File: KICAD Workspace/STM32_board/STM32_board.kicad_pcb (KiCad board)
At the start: 2 copper layers, 171.4 x 151.8 mm, 25 parts, among them J1 Power connector, J10 Low side connector, J2 High side connector, J3 Sensors connector, J4 LCD interface, J5 Low side connector, J6 3v3_out, J7 Joystick connector, J9 UART module, U1 CD4050BE, U2 LM7805_TO220, U3 LP2950-3.3_TO92

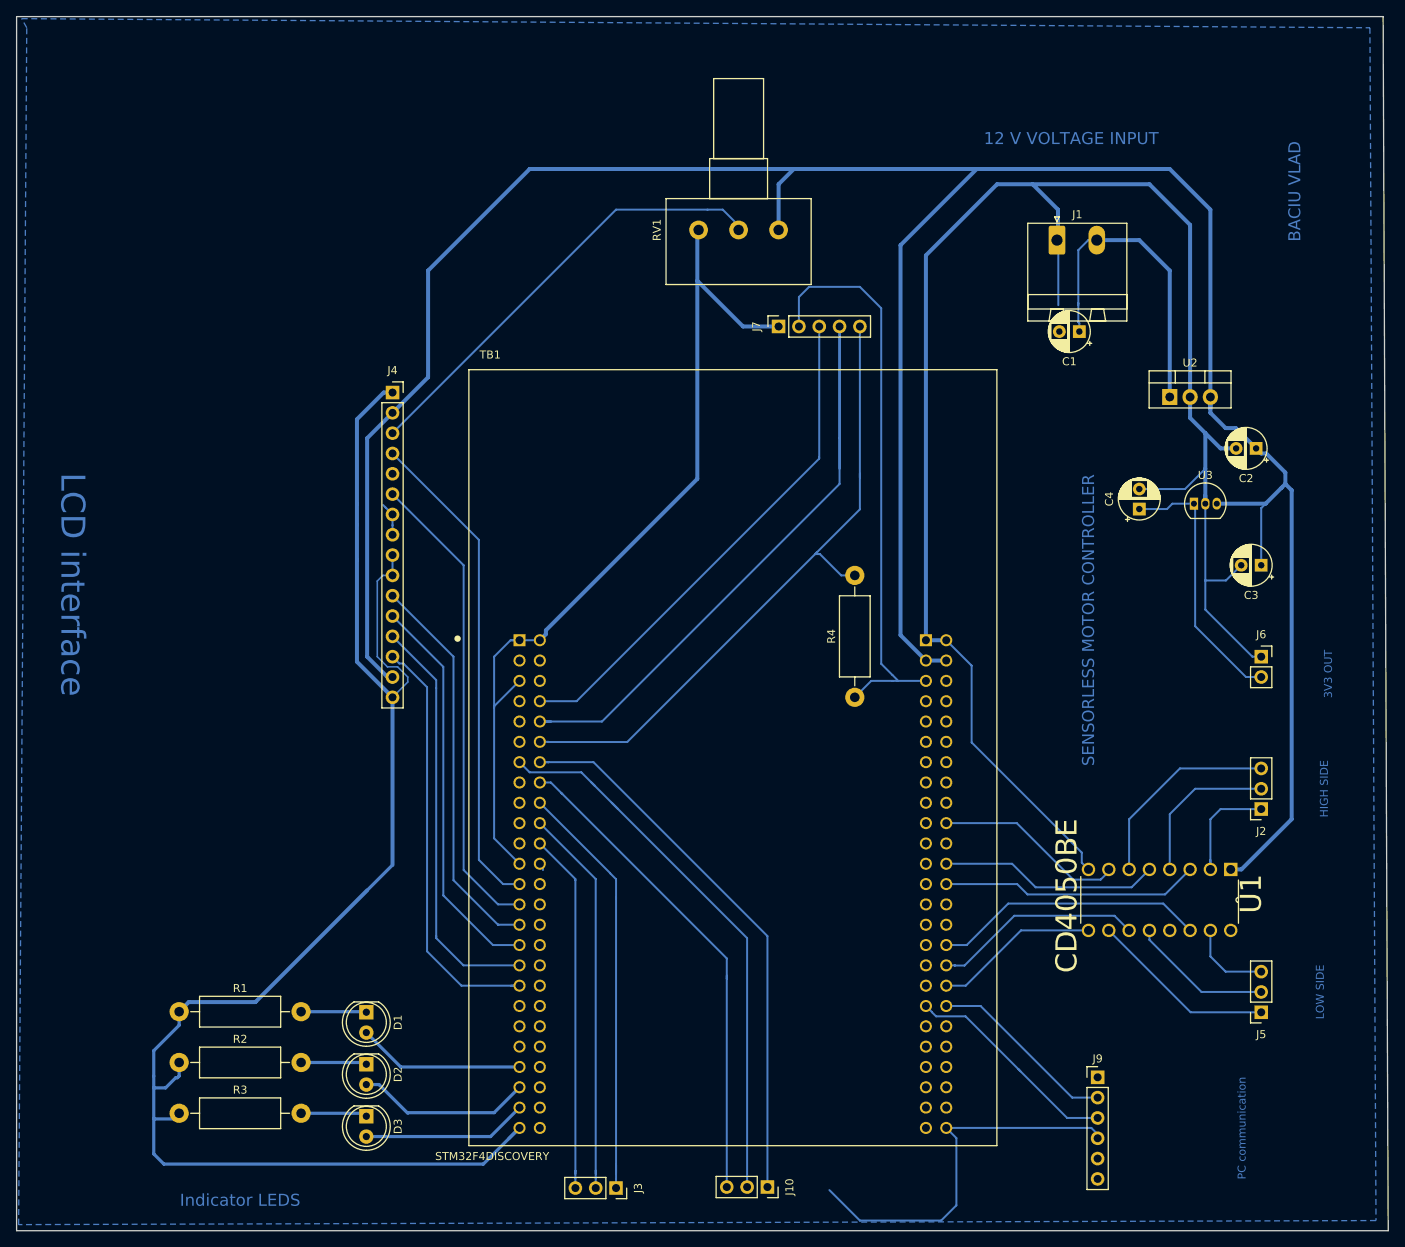
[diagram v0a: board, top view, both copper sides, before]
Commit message: Final version for printing (i hope)
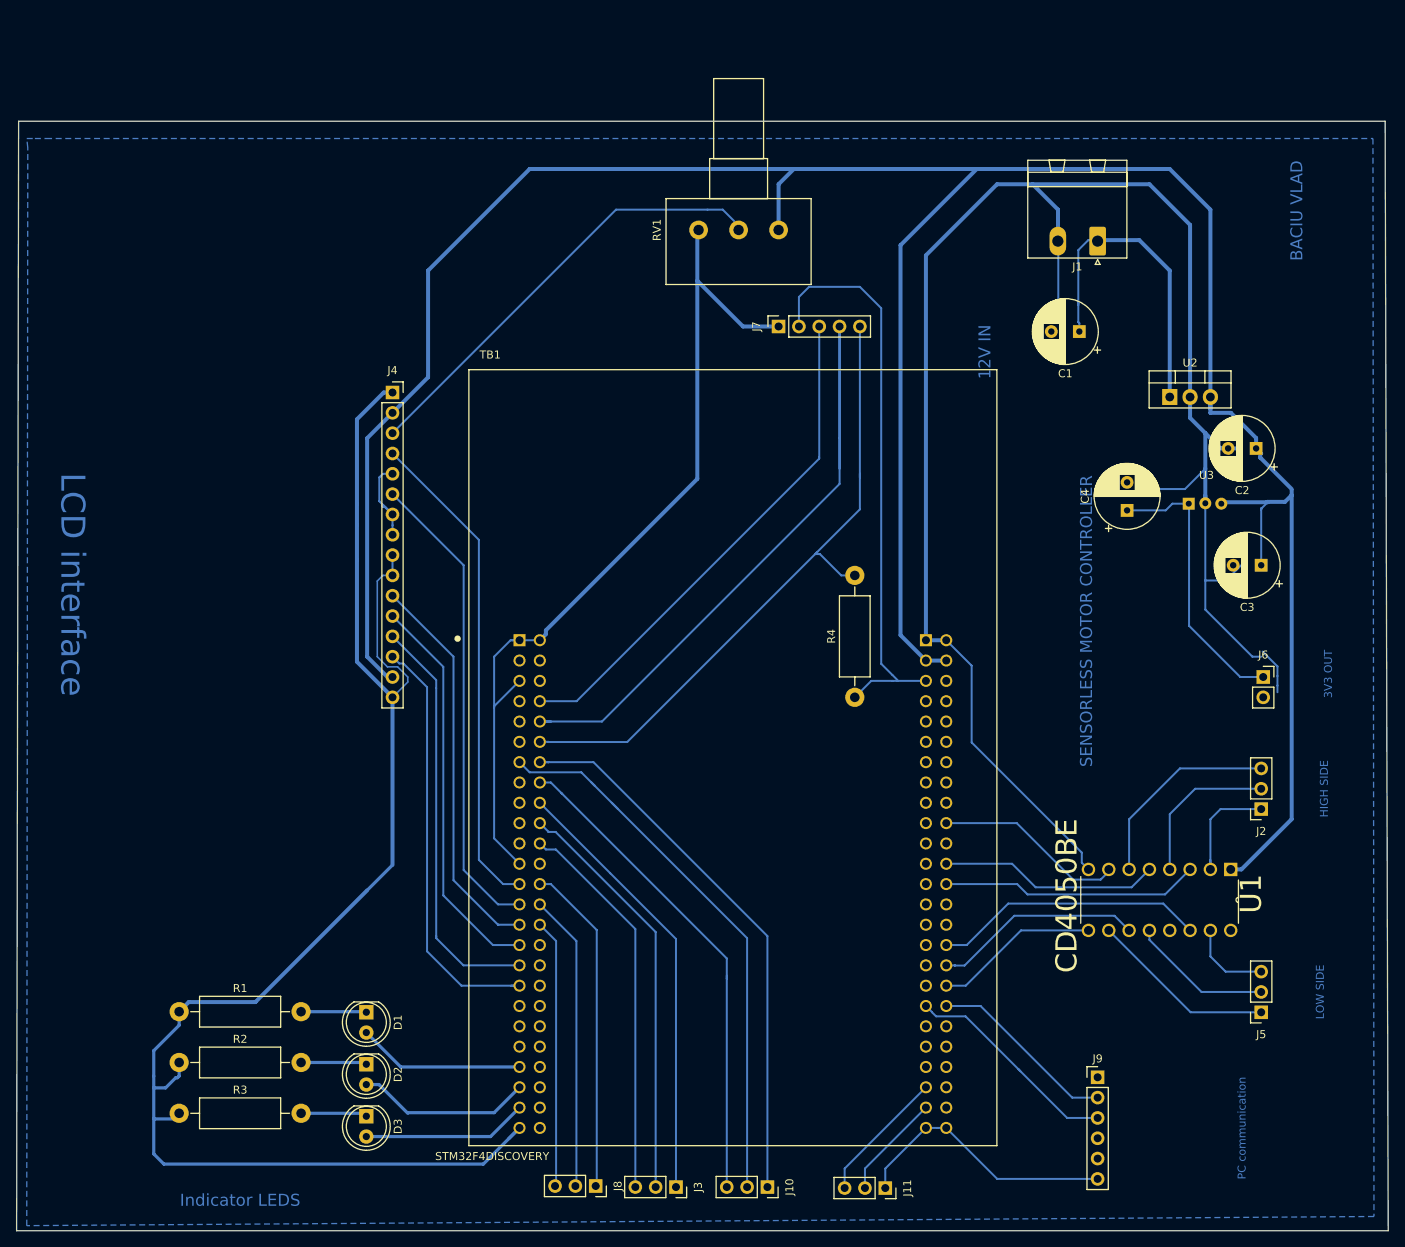
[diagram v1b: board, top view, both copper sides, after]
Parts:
- added J11: Output pins, Connector_PinSocket_2.54mm:PinSocket_1x03_P2.54mm_Vertical, F.Cu at (126.0, 160.4)
- added J8: Output pins, Connector_PinSocket_2.54mm:PinSocket_1x03_P2.54mm_Vertical, F.Cu at (89.8, 160.1)
- C1, C2, C3, C4: footprint Capacitor_THT:CP_Radial_D5.0mm_P2.50mm -> Capacitor_THT:CP_Radial_D8.0mm_P3.50mm
- moved J3 7.49 mm to (99.8, 160.3)
- moved J1 5.08 mm to (152.5, 42.0), turned to 180 degrees
- moved J6 2.55 mm to (173.2, 96.5)
- moved C4 1.53 mm to (156.2, 75.7)
- moved U3 0.15 mm to (164.9, 74.9)
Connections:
- J1 pad 1: /GND -> /12V
- J1 pad 2: /12V -> /GND
- J6 pad 1: /GND -> /3V3
- J6 pad 2: /3V3 -> /GND
- TB1 pad P1_24: /EXT_4 -> Net-(TB1-PadP1_24)
- TB1 pad P2_45: Net-(TB1-PadP2_45) -> /EXT_3
- TB1 pad P2_47: Net-(TB1-PadP2_47) -> /EXT_4
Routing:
- net /EXT_5: track 0.00 -> 41.4 mm
- net /EXT_6: track 0.00 -> 37.0 mm
- net /EXT_7: track 0.00 -> 33.4 mm
- net /EXT_3: track 0.00 -> 17.1 mm
- net /EXT_4: track 1.34 -> 13.5 mm
- net /READ_BATTERY: track 45.3 -> 48.6 mm
- net /ADC_BATTERY: track 49.1 -> 52.2 mm
- net /3V3: track 33.3 -> 35.7 mm
- net /CURRENT_SENSOR: track 53.4 -> 55.1 mm
- net /5V: track 353.4 -> 351.9 mm
- net /GND: track 622.6 -> 624.0 mm
- net Net-(TB1-PadP1_24): track 0.00 -> 0.94 mm
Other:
- board size 171.4 x 151.8 mm -> 171.4 x 138.7 mm
- board text added: "12V IN"
- board text removed: "12 V VOLTAGE INPUT"
